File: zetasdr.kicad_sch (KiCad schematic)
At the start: 46 parts, among them J1 Output I, J2 USB_B, J3 Output Q, J4 Input AWG, J5 Antenna, Q1 BC547C, U1 74AHC1G04, U2 74HC74, U3 4052, U4 NE5532

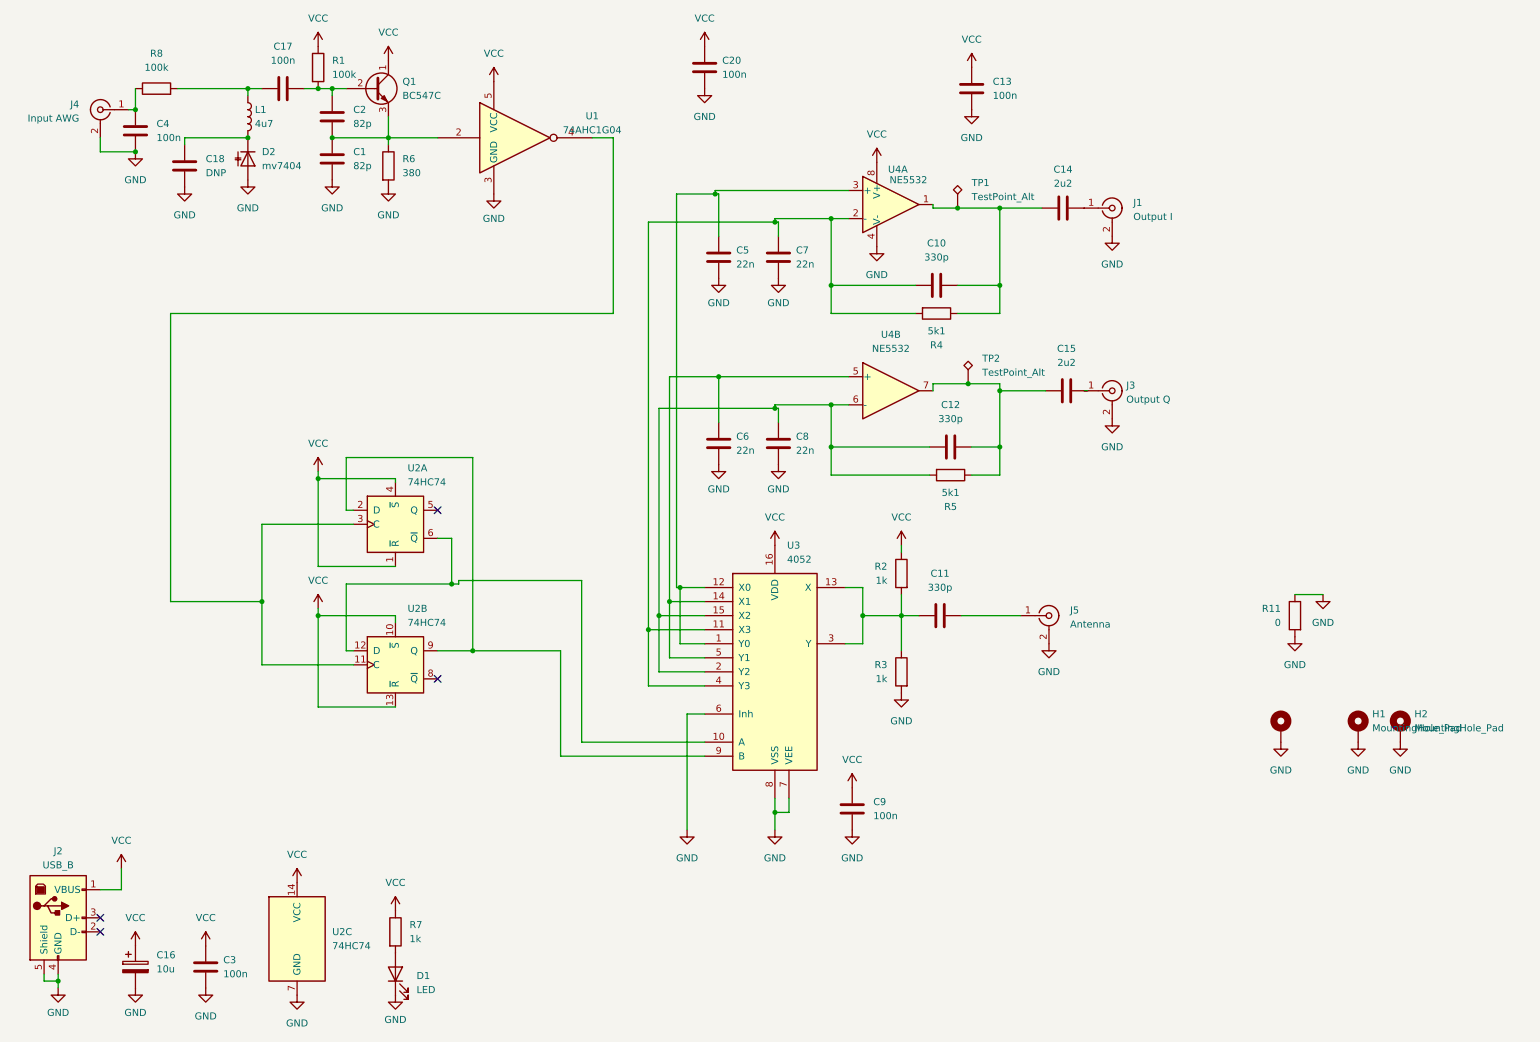
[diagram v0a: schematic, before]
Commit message: first layout
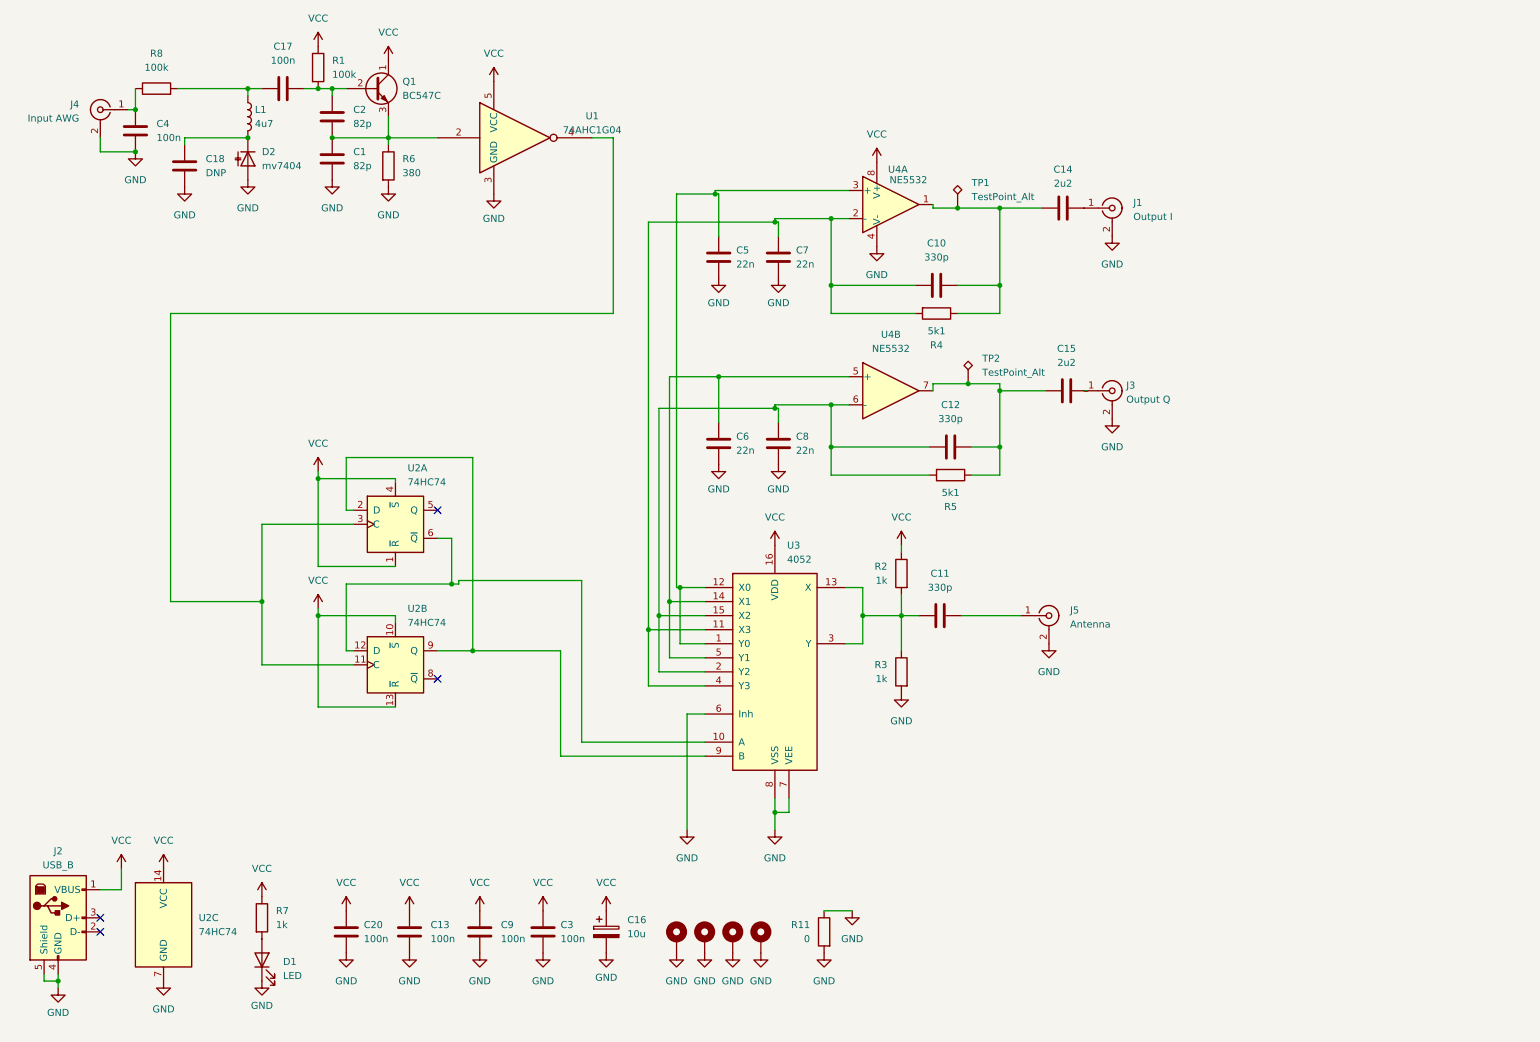
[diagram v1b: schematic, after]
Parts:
- added H3: MountingHole_Pad, MountingHole:MountingHole_3.2mm_M3_Pad, symbol Mechanical:MountingHole_Pad
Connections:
- net GND: now also H3.1
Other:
- moved on the sheet: C13, C16, C20, C3, C9, D1, R11, R7, U2C
